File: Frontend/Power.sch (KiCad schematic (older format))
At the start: 27 parts, among them J11 APWR, U23 LM317S, U24 MCP9700T-E/TT, U25 L78M05CDT, U26 TLV70233DSE, U27 MCP9700T-E/TT, U28 MC79M05CDT

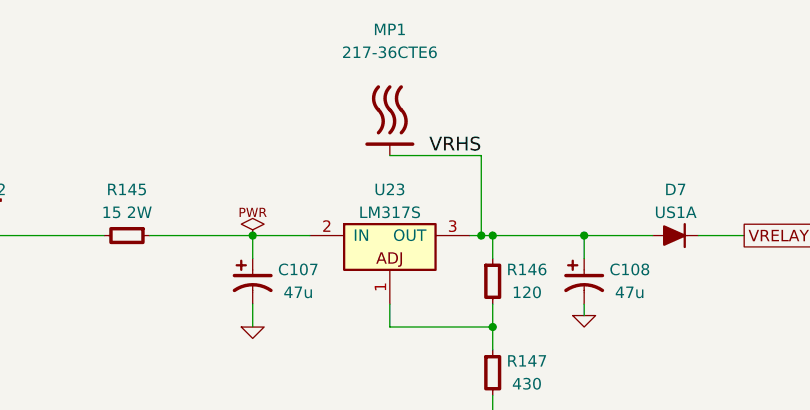
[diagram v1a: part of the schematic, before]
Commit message: Even more layout tweaks
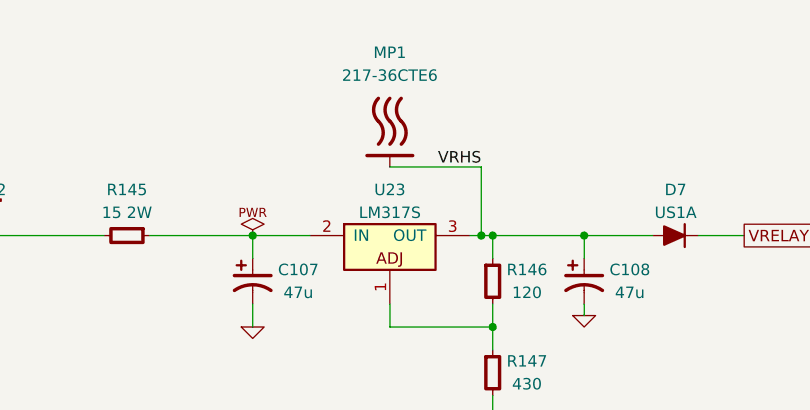
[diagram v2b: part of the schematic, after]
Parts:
- E4, E5: BOM DIST DIGIKEY 732-1622-1-ND -> BEAD SMD 120 1A [1206]
- MP1: BOM (none) -> DIST DIGIKEY 345-1099-ND; Manuf (none) -> Wakefield; PN (none) -> 217-36CTE6
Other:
- moved on the sheet: MP1
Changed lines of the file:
@@
 $EndComp
 $Comp
-L GND #PWR0338
+L GND #PWR0340
 U 1 1 552FAC91
 P 2700 5400
-F 0 "#PWR0338" H 2700 5400 30  0001 C CNN
+F 0 "#PWR0340" H 2700 5400 30  0001 C CNN
 F 1 "GND" H 2700 5330 30  0001 C CNN
 F 2 "" H 2700 5400 60  0000 C CNN
@@
 $EndComp
 $Comp
-L GND #PWR0339
+L GND #PWR0341
 U 1 1 552FB1F9
 P 3300 5400
-F 0 "#PWR0339" H 3300 5400 30  0001 C CNN
+F 0 "#PWR0341" H 3300 5400 30  0001 C CNN
 F 1 "GND" H 3300 5330 30  0001 C CNN
 F 2 "" H 3300 5400 60  0000 C CNN
@@
 $EndComp
 $Comp
-L GND #PWR0340
+L GND #PWR0342
 U 1 1 552FBBCC
 P 4250 5400
-F 0 "#PWR0340" H 4250 5400 30  0001 C CNN
+F 0 "#PWR0342" H 4250 5400 30  0001 C CNN
 F 1 "GND" H 4250 5330 30  0001 C CNN
 F 2 "" H 4250 5400 60  0000 C CNN
@@
 $EndComp
 $Comp
-L GND #PWR0341
+L GND #PWR0343
 U 1 1 552FBE04
 P 4700 5400
-F 0 "#PWR0341" H 4700 5400 30  0001 C CNN
+F 0 "#PWR0343" H 4700 5400 30  0001 C CNN
 F 1 "GND" H 4700 5330 30  0001 C CNN
 F 2 "" H 4700 5400 60  0000 C CNN
@@
 $EndComp
 $Comp
-L -5 #PWR0342
+L -5 #PWR0344
 U 1 1 552FBF15
 P 4700 4950
-F 0 "#PWR0342" H 4700 4900 30  0001 C CNN
+F 0 "#PWR0344" H 4700 4900 30  0001 C CNN
 F 1 "-5" H 4700 4850 50  0000 C CNN
 F 2 "" H 4700 4950 60  0000 C CNN
@@
 $EndComp
 $Comp
-L GND #PWR0343
+L GND #PWR0345
 U 1 1 552FD87A
 P 5100 3250
-F 0 "#PWR0343" H 5100 3250 30  0001 C CNN
+F 0 "#PWR0345" H 5100 3250 30  0001 C CNN
 F 1 "GND" H 5100 3180 30  0001 C CNN
 F 2 "" H 5100 3250 60  0000 C CNN
@@
 $EndComp
 $Comp
-L +12 #PWR0344
+L +12 #PWR0346
 U 1 1 5530425A
 P 2500 2800
-F 0 "#PWR0344" H 2500 2850 30  0001 C CNN
+F 0 "#PWR0346" H 2500 2850 30  0001 C CNN
 F 1 "+12" H 2500 2900 50  0000 C CNN
 F 2 "" H 2500 2800 60  0000 C CNN
@@
 Connection ~ 4700 3300
 $Comp
-L GND #PWR0345
+L GND #PWR0347
 U 1 1 5547D09D
 P 4700 3700
-F 0 "#PWR0345" H 4700 3700 30  0001 C CNN
+F 0 "#PWR0347" H 4700 3700 30  0001 C CNN
 F 1 "GND" H 4700 3630 30  0001 C CNN
 F 2 "" H 4700 3700 60  0000 C CNN
@@
 Connection ~ 3650 2900
 $Comp
-L GND #PWR0346
+L GND #PWR0348
 U 1 1 55480232
 P 3650 3300
-F 0 "#PWR0346" H 3650 3300 30  0001 C CNN
+F 0 "#PWR0348" H 3650 3300 30  0001 C CNN
 F 1 "GND" H 3650 3230 30  0001 C CNN
 F 2 "" H 3650 3300 60  0000 C CNN
@@
 	4700 4300 4700 4400
 $Comp
-L +5 #PWR0347
+L +5 #PWR0349
 U 1 1 55480B1F
 P 4800 4250
-F 0 "#PWR0347" H 4800 4300 30  0001 C CNN
+F 0 "#PWR0349" H 4800 4300 30  0001 C CNN
 F 1 "+5" H 4800 4350 50  0000 C CNN
 F 2 "" H 4800 4250 60  0000 C CNN
@@
 Connection ~ 4700 4300
 $Comp
-L GND #PWR0348
+L GND #PWR0350
 U 1 1 55480BB8
 P 4250 4650
-F 0 "#PWR0348" H 4250 4650 30  0001 C CNN
+F 0 "#PWR0350" H 4250 4650 30  0001 C CNN
 F 1 "GND" H 4250 4580 30  0001 C CNN
 F 2 "" H 4250 4650 60  0000 C CNN
@@
 	4250 4650 4250 4600
 $Comp
-L GND #PWR0349
+L GND #PWR0351
 U 1 1 55480C51
 P 4700 4650
-F 0 "#PWR0349" H 4700 4650 30  0001 C CNN
+F 0 "#PWR0351" H 4700 4650 30  0001 C CNN
 F 1 "GND" H 4700 4580 30  0001 C CNN
 F 2 "" H 4700 4650 60  0000 C CNN
@@
 	1800 4300 3900 4300
 $Comp
-L +8 #PWR0350
+L +8 #PWR0352
 U 1 1 55480F09
 P 2600 4250
-F 0 "#PWR0350" H 2600 4300 30  0001 C CNN
+F 0 "#PWR0352" H 2600 4300 30  0001 C CNN
 F 1 "+8" H 2600 4350 50  0000 C CNN
 F 2 "" H 2600 4250 60  0000 C CNN
@@
 Connection ~ 3300 4300
 $Comp
-L GND #PWR0351
+L GND #PWR0353
 U 1 1 55481C45
 P 3300 4650
-F 0 "#PWR0351" H 3300 4650 30  0001 C CNN
+F 0 "#PWR0353" H 3300 4650 30  0001 C CNN
 F 1 "GND" H 3300 4580 30  0001 C CNN
 F 2 "" H 3300 4650 60  0000 C CNN
@@
 Connection ~ 2700 4300
 $Comp
-L GND #PWR0352
+L GND #PWR0354
 U 1 1 55481E79
 P 2700 4650
-F 0 "#PWR0352" H 2700 4650 30  0001 C CNN
+F 0 "#PWR0354" H 2700 4650 30  0001 C CNN
 F 1 "GND" H 2700 4580 30  0001 C CNN
 F 2 "" H 2700 4650 60  0000 C CNN
@@
 	2700 4650 2700 4600
 $Comp
-L -8 #PWR0353
+L -8 #PWR0355
 U 1 1 55482517
 P 2600 4950
-F 0 "#PWR0353" H 2600 4900 30  0001 C CNN
+F 0 "#PWR0355" H 2600 4900 30  0001 C CNN
 F 1 "-8" H 2600 4850 50  0000 C CNN
 F 2 "" H 2600 4950 60  0000 C CNN
@@
 F 4 "742792113" H 1700 4300 60  0001 C CNN "PN"
 F 5 "Wurth" H 1700 4300 60  0001 C CNN "Manuf"
-F 6 "DIST DIGIKEY 732-1622-1-ND" H 1700 4300 60  0001 C CNN "BOM"
+F 6 "BEAD SMD 120 1A [1206]" H 1700 4300 60  0001 C CNN "BOM"
 	1    1700 4300
 	1    0    0    -1
@@
 F 4 "742792113" H 1700 4600 60  0001 C CNN "PN"
 F 5 "Wurth" H 1700 4600 60  0001 C CNN "Manuf"
-F 6 "DIST DIGIKEY 732-1622-1-ND" H 1700 4600 60  0001 C CNN "BOM"
+F 6 "BEAD SMD 120 1A [1206]" H 1700 4600 60  0001 C CNN "BOM"
 	1    1700 4600
 	1    0    0    -1
@@
 	2700 5000 2700 5100
 $Comp
-L GND #PWR0354
+L GND #PWR0356
 U 1 1 55483EF7
 P 1500 4750
-F 0 "#PWR0354" H 1500 4750 30  0001 C CNN
+F 0 "#PWR0356" H 1500 4750 30  0001 C CNN
 F 1 "GND" H 1500 4680 30  0001 C CNN
 F 2 "" H 1500 4750 60  0000 C CNN
@@
 Connection ~ 4800 4300
 $Comp
-L GND #PWR0355
+L GND #PWR0357
 U 1 1 555465A7
 P 6500 4550
-F 0 "#PWR0355" H 6500 4550 30  0001 C CNN
+F 0 "#PWR0357" H 6500 4550 30  0001 C CNN
 F 1 "GND" H 6500 4480 30  0001 C CNN
 F 2 "" H 6500 4550 60  0000 C CNN
@@
 Connection ~ 5200 4300
 $Comp
-L GND #PWR0356
+L GND #PWR0358
 U 1 1 55548553
 P 5200 4650
-F 0 "#PWR0356" H 5200 4650 30  0001 C CNN
+F 0 "#PWR0358" H 5200 4650 30  0001 C CNN
 F 1 "GND" H 5200 4580 30  0001 C CNN
 F 2 "" H 5200 4650 60  0000 C CNN
@@
 	6700 4300 6700 4400
 $Comp
-L GND #PWR0357
+L GND #PWR0359
 U 1 1 5554875C
 P 6700 4650
-F 0 "#PWR0357" H 6700 4650 30  0001 C CNN
+F 0 "#PWR0359" H 6700 4650 30  0001 C CNN
 F 1 "GND" H 6700 4580 30  0001 C CNN
 F 2 "" H 6700 4650 60  0000 C CNN
@@
 L HEATSINK-CONN MP1
 U 1 1 55503A38
-P 4250 2450
+P 4250 2500
 F 0 "MP1" H 4250 2900 50  0000 C CNN
 F 1 "217-36CTE6" H 4250 2800 50  0000 C CNN
-F 2 "manuf:LAIRD-BMI-S-203" H 4250 2450 60  0001 C CNN
-F 3 "" H 4250 2450 60  0000 C CNN
-	1    4250 2450
-	1    0    0    -1
-$EndComp
-Wire Wire Line
-	4250 2550 4650 2550
-Wire Wire Line
-	4650 2550 4650 2900
+F 2 "manuf:LAIRD-BMI-S-203" H 4250 2500 60  0001 C CNN
+F 3 "" H 4250 2500 60  0000 C CNN
+F 4 "217-36CTE6" H 4250 2500 60  0001 C CNN "PN"
+F 5 "Wakefield" H 4250 2500 60  0001 C CNN "Manuf"
+F 6 "DIST DIGIKEY 345-1099-ND" H 4250 2500 60  0001 C CNN "BOM"
+	1    4250 2500
+	1    0    0    -1
+$EndComp
+Wire Wire Line
+	4250 2600 4650 2600
+Wire Wire Line
+	4650 2600 4650 2900
 Connection ~ 4650 2900
-Text Label 4650 2550 2    60   ~ 0
+Text Label 4650 2600 2    50   ~ 0
 VRHS
 $Comp
@@
 $EndComp
 $Comp
-L +3.3 #PWR0358
+L +3.3 #PWR0360
 U 1 1 555461CC
 P 8050 3150
-F 0 "#PWR0358" H 8050 3200 30  0001 C CNN
+F 0 "#PWR0360" H 8050 3200 30  0001 C CNN
 F 1 "+3.3" H 8050 3250 50  0000 C CNN
 F 2 "" H 8050 3150 60  0000 C CNN
@@
 	8050 3200 8100 3200
 $Comp
-L GND #PWR0359
+L GND #PWR0361
 U 1 1 55546814
 P 8050 3450
-F 0 "#PWR0359" H 8050 3450 30  0001 C CNN
+F 0 "#PWR0361" H 8050 3450 30  0001 C CNN
 F 1 "GND" H 8050 3380 30  0001 C CNN
 F 2 "" H 8050 3450 60  0000 C CNN
@@
 $EndComp
 $Comp
-L +3.3 #PWR0360
+L +3.3 #PWR0362
 U 1 1 5554715F
 P 7700 3150
-F 0 "#PWR0360" H 7700 3200 30  0001 C CNN
+F 0 "#PWR0362" H 7700 3200 30  0001 C CNN
 F 1 "+3.3" H 7700 3250 50  0000 C CNN
 F 2 "" H 7700 3150 60  0000 C CNN
@@
 	7700 3200 7700 3150
 $Comp
-L GND #PWR0361
+L GND #PWR0363
 U 1 1 55547208
 P 7700 3450
-F 0 "#PWR0361" H 7700 3450 30  0001 C CNN
+F 0 "#PWR0363" H 7700 3450 30  0001 C CNN
 F 1 "GND" H 7700 3380 30  0001 C CNN
 F 2 "" H 7700 3450 60  0000 C CNN
@@
 $EndComp
 $Comp
-L +3.3 #PWR0362
+L +3.3 #PWR0364
 U 1 1 555474B3
 P 8050 4250
-F 0 "#PWR0362" H 8050 4300 30  0001 C CNN
+F 0 "#PWR0364" H 8050 4300 30  0001 C CNN
 F 1 "+3.3" H 8050 4350 50  0000 C CNN
 F 2 "" H 8050 4250 60  0000 C CNN
@@
 	8050 4300 8100 4300
 $Comp
-L GND #PWR0363
+L GND #PWR0365
 U 1 1 555474BB
 P 8050 4550
-F 0 "#PWR0363" H 8050 4550 30  0001 C CNN
+F 0 "#PWR0365" H 8050 4550 30  0001 C CNN
 F 1 "GND" H 8050 4480 30  0001 C CNN
 F 2 "" H 8050 4550 60  0000 C CNN
@@
 $EndComp
 $Comp
-L +3.3 #PWR0364
+L +3.3 #PWR0366
 U 1 1 555474CB
 P 7700 4250
-F 0 "#PWR0364" H 7700 4300 30  0001 C CNN
+F 0 "#PWR0366" H 7700 4300 30  0001 C CNN
 F 1 "+3.3" H 7700 4350 50  0000 C CNN
 F 2 "" H 7700 4250 60  0000 C CNN
@@
 	7700 4300 7700 4250
 $Comp
-L GND #PWR0365
+L GND #PWR0367
 U 1 1 555474D2
 P 7700 4550
-F 0 "#PWR0365" H 7700 4550 30  0001 C CNN
+F 0 "#PWR0367" H 7700 4550 30  0001 C CNN
 F 1 "GND" H 7700 4480 30  0001 C CNN
 F 2 "" H 7700 4550 60  0000 C CNN
@@
 	5600 4400 5700 4400
 $Comp
-L +3.3 #PWR0366
+L +3.3 #PWR0368
 U 1 1 55545BBA
 P 5600 3900
-F 0 "#PWR0366" H 5600 3950 30  0001 C CNN
+F 0 "#PWR0368" H 5600 3950 30  0001 C CNN
 F 1 "+3.3" H 5600 4000 50  0000 C CNN
 F 2 "" H 5600 3900 60  0000 C CNN
@@
 The analog 3.3V rail is enabled by the digital 3.3V rail, so the\nDAC is not powered if separate analog power cable is\ndisconnected. @R148 forms a low-pass filter with the input and\noutput capacitors to prevent injection of noise from the digital rail.
 $Comp
-L PWR #PWR0367
+L PWR #PWR0369
 U 1 1 55580BE7
 P 2000 4250
-F 0 "#PWR0367" H 2000 4250 50  0001 C CNN
+F 0 "#PWR0369" H 2000 4250 50  0001 C CNN
 F 1 "PWR" H 2000 4250 50  0001 C CNN
 F 2 "" H 2000 4250 60  0000 C CNN
@@
 Connection ~ 2000 4300
 $Comp
-L PWR #PWR0368
+L PWR #PWR0370
 U 1 1 55580C88
 P 2000 4550
-F 0 "#PWR0368" H 2000 4550 50  0001 C CNN
+F 0 "#PWR0370" H 2000 4550 50  0001 C CNN
 F 1 "PWR" H 2000 4550 50  0001 C CNN
 F 2 "" H 2000 4550 60  0000 C CNN
@@
 Connection ~ 2000 4600
 $Comp
-L PWR #PWR0369
+L PWR #PWR0371
 U 1 1 55587045
 P 3650 2900
-F 0 "#PWR0369" H 3650 2900 50  0001 C CNN
+F 0 "#PWR0371" H 3650 2900 50  0001 C CNN
 F 1 "PWR" H 3650 2900 50  0001 C CNN
 F 2 "" H 3650 2900 60  0000 C CNN
